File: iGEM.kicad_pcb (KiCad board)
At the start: 4 copper layers, 81.1 x 56.1 mm, 50 parts, among them IC1 TMCS1107A1BQDRQ1, IC2 TMCS1107A1BQDRQ1, IC3 MCP4642-502E_UN, J1 Conn_01x02, J2 Conn_01x02, J3 Conn_01x02, J4 Conn_01x03, M1 Fan, Q1 TIP122, Q2 TIP122, Q3 IRF4905, Q4 D44VH, Q5 IRF4905, Q6 D44VH, U1 ADC101C021CIMK, U2 ADC101C021CIMK, U3 PCA9536D, U4 ICL7667

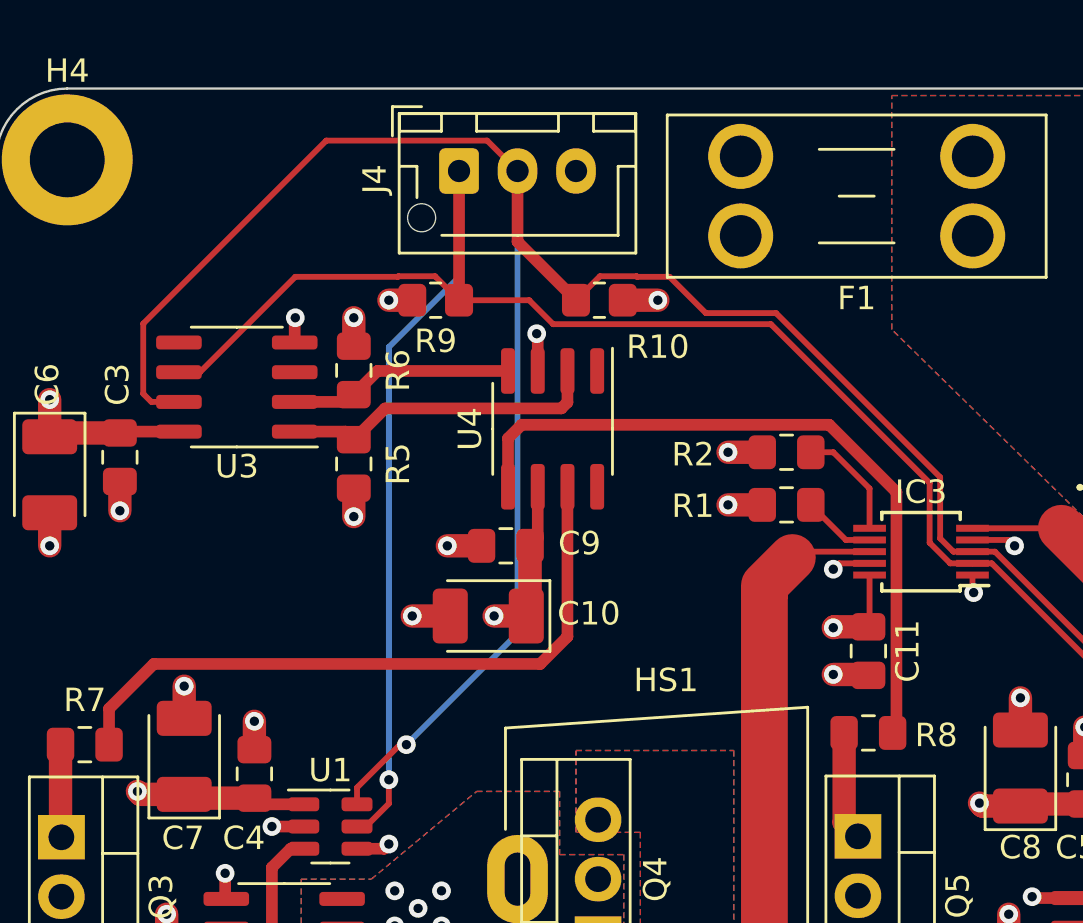
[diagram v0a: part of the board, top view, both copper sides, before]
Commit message: layout cleanup
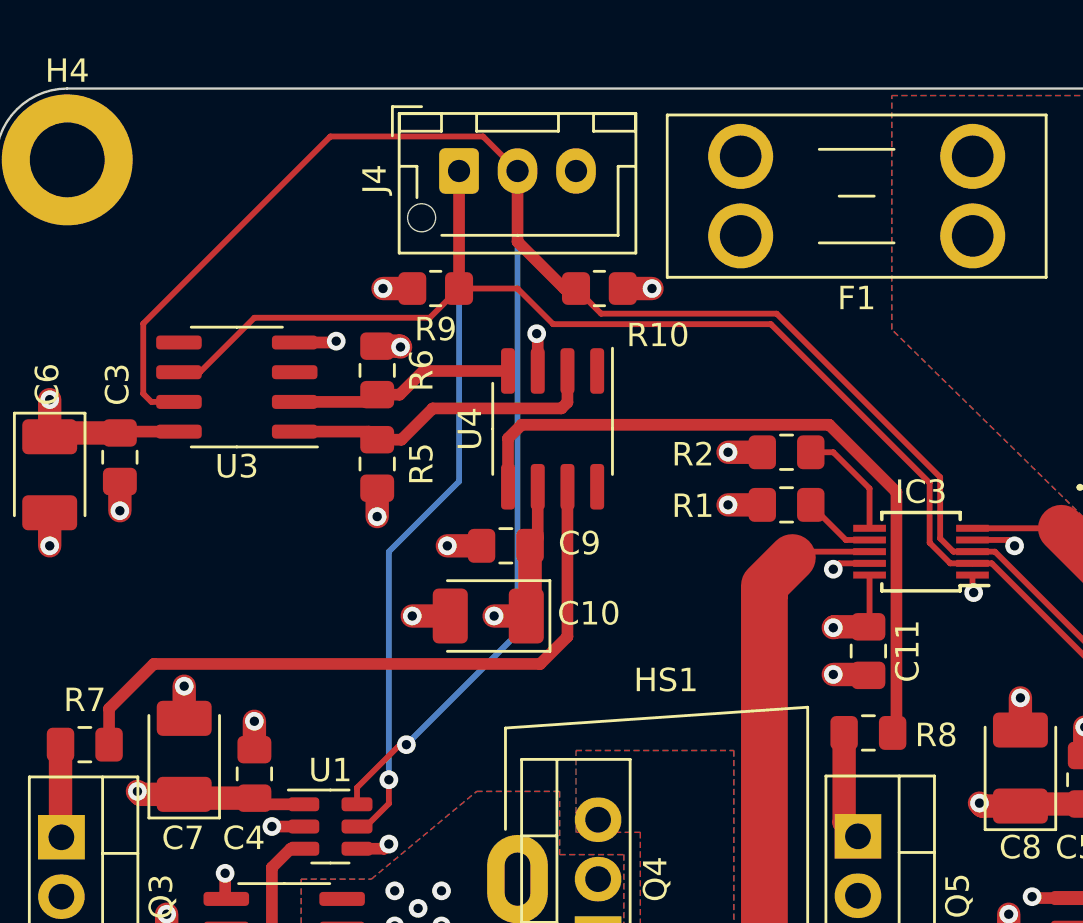
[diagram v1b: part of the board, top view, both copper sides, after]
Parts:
- moved R5 1.00 mm to (138.5, 55.0)
- moved R6 1.00 mm to (138.5, 51.0)
- moved R10 0.50 mm to (148.0, 47.5)
- moved R9 0.50 mm to (141.0, 47.5)
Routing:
- net SCL: track 93.7 -> 92.7 mm
- net SDA: track 100.1 -> 99.4 mm
- net GND: track 31.4 -> 31.9 mm
